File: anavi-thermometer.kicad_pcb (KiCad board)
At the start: 2 copper layers, 74.9 x 40.6 mm, 25 parts, among them P1 CONN_01X03, SW1 SW_DIP_x01, U1 I2C_SENS_1, U2 I2C_SENS_1, U3 I2C_SENS_1, U4 Conn_01x04

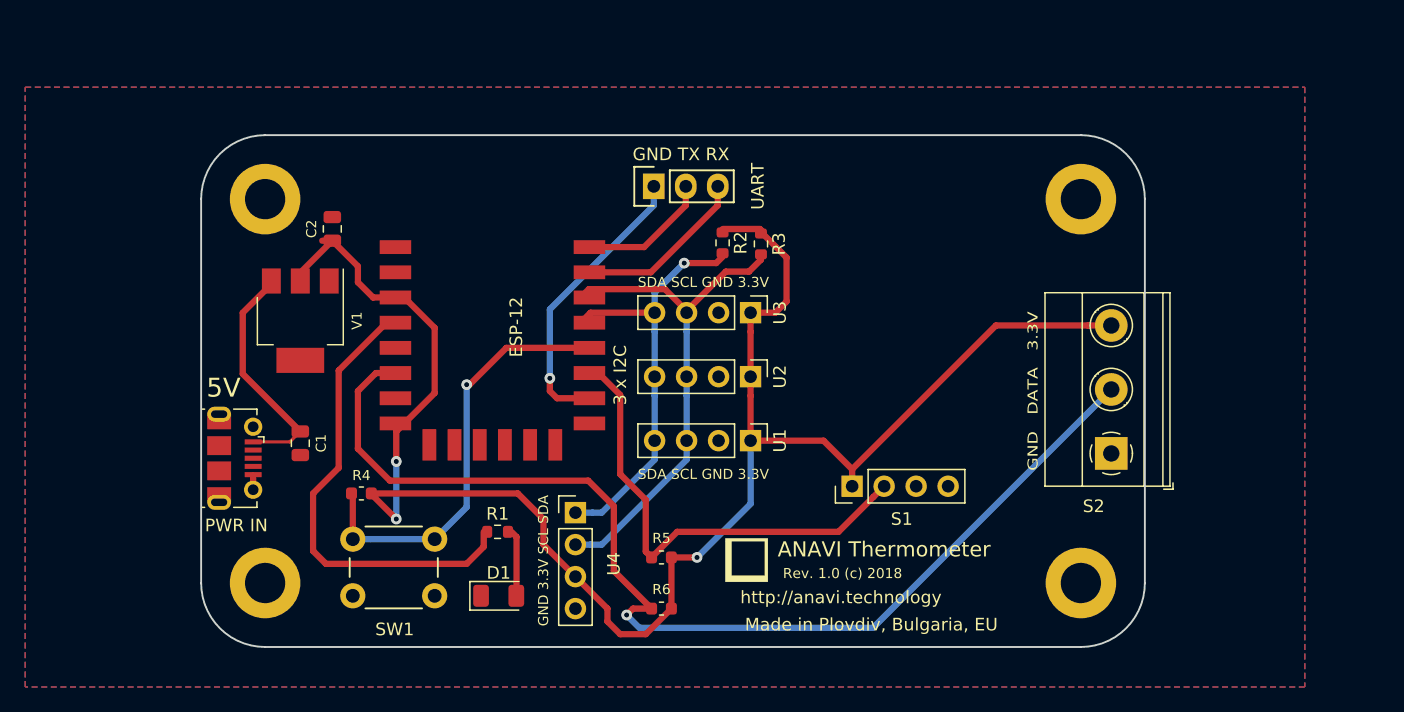
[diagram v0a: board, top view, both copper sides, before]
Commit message: rev 0.1
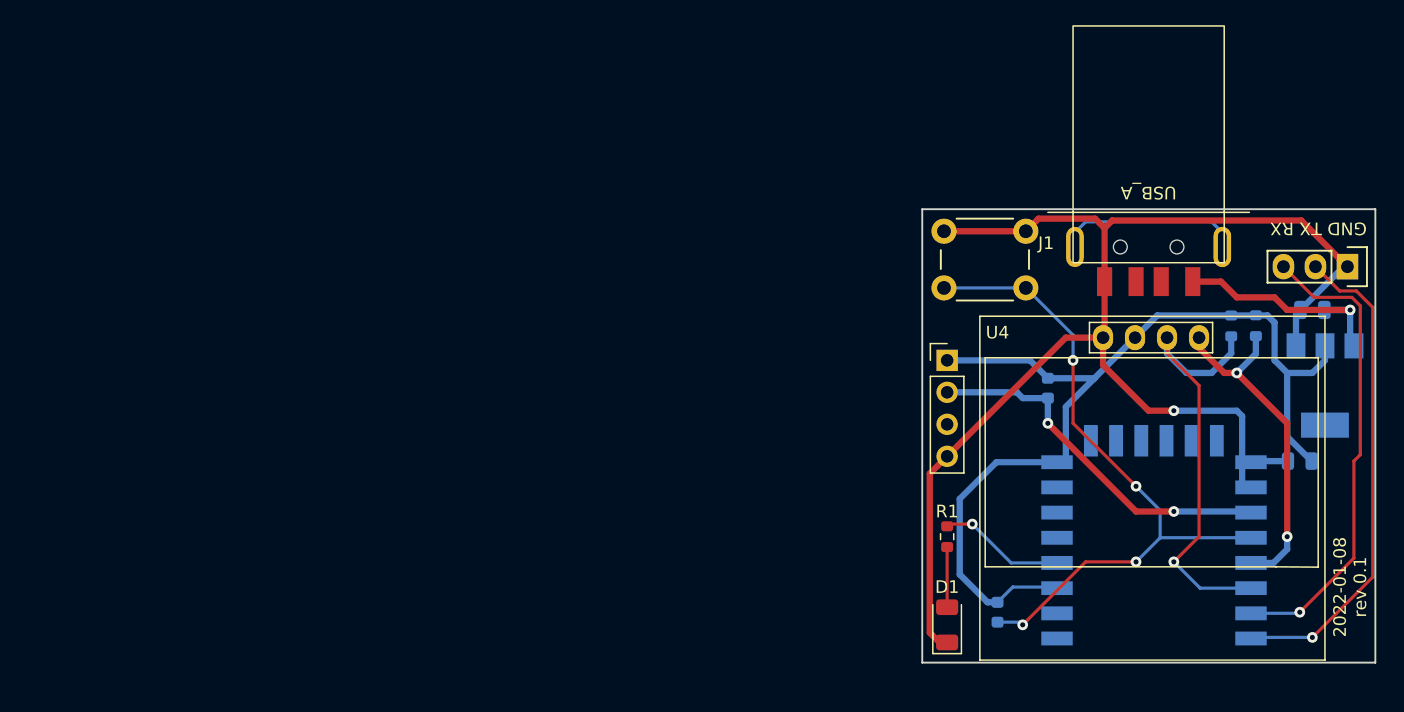
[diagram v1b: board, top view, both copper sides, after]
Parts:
- removed G***: LOGO, logo:anavi-logo
- removed PWR IN: USB_B_Micro, Connector_USB:USB_Micro-B_Molex-105017-0001
- removed R6: 4,7K, Resistor_SMD:R_0603_1608Metric
- removed REF** (x4): MountingHole_3.2mm_M3_DIN965_Pad, Mounting_Holes:MountingHole_3.2mm_M3_DIN965_Pad
- removed S2: DS18B20, TerminalBlock_Phoenix:TerminalBlock_Phoenix_MKDS-1,5-3-5.08_1x03_P5.08mm_Horizontal
- removed U1, U2, U3: I2C_SENS_1, Connector_PinHeader_2.54mm:PinHeader_1x04_P2.54mm_Vertical
- added J1: USB_A, GCT_USB1061_Horizontal:USB_A_Plug_GCT_USB1061_Horizontal, F.Cu at (140.0, 80.0)
- C1, C2, ESP-12, R2, R3, R4, R5, V1: moved to B.Cu
- U4: value Conn_01x04 -> SSD1306; footprint Connector_PinHeader_2.54mm:PinHeader_1x04_P2.54mm_Vertical -> SSD1306:128x64OLED
- moved V1 81.5 mm to (154.0, 91.0)
- moved C1 81.0 mm to (153.0, 85.0), turned to 180 degrees
- moved C2 79.0 mm to (152.0, 97.0), turned to 180 degrees
- moved ESP-12 61.0 mm to (133.4, 111.1)
- moved P1 55.4 mm to (155.8, 81.6), turned to -90 degrees
- moved R4 51.4 mm to (128.0, 109.0), turned to 90 degrees
- moved SW1 49.7 mm to (123.8, 78.8), turned to 0 degrees
- moved U4 45.6 mm to (140.0, 97.8)
- moved R2 42.9 mm to (148.5, 86.3)
- moved R3 37.9 mm to (146.6, 86.3)
- moved R1 35.7 mm to (124.0, 103.0), turned to -90 degrees
- moved D1 35.7 mm to (124.0, 110.0), turned to 90 degrees
- moved R5 33.5 mm to (132.0, 91.2), turned to -90 degrees
- moved S1 12.5 mm to (124.0, 89.0), turned to 0 degrees
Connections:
- ESP-12 pad 6: Net-(ESP-12-Pad6) -> unconnected-(ESP-12-Pad6)
- U4 pad 1: Net-(ESP-12-Pad13) -> GND
- U4 pad 2: Net-(ESP-12-Pad14) -> +3V3
- U4 pad 3: +3V3 -> Net-(ESP-12-Pad14)
- U4 pad 4: GND -> Net-(ESP-12-Pad13)
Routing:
- net Net-(ESP-12-Pad6): track 89.4 -> 0.00 mm, vias 1 -> 0
- net GND: track 23.5 -> 108.2 mm
- net +3V3: track 143.2 -> 78.8 mm, vias 3 -> 0
- net Net-(ESP-12-Pad16): track 11.2 -> 39.7 mm, vias 0 -> 1
- net Net-(ESP-12-Pad4): track 37.7 -> 10.8 mm, vias 0 -> 1
- net Net-(ESP-12-Pad15): track 14.6 -> 38.3 mm, vias 0 -> 1
- net Net-(ESP-12-Pad12): track 33.7 -> 53.1 mm, vias 2 -> 4
- net unconnected-(J1-Pad5): track 0.00 -> 14.7 mm
- net Net-(ESP-12-Pad11): track 38.6 -> 28.6 mm, vias 0 -> 2
- net Net-(ESP-12-Pad13): track 34.4 -> 27.9 mm, vias 1 -> 2
- net Net-(ESP-12-Pad14): track 40.6 -> 35.0 mm, vias 0 -> 1
- net +5V: track 19.4 -> 18.5 mm, vias 0 -> 1
- removed copper zone on B.Cu, net GND
- removed copper zone on F.Cu, net GND
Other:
- board size 74.9 x 40.6 mm -> 36 x 36 mm
- board text added: "2022-01-08 rev 0.1"
- board text added: "3V3"
- board text added: "DAT"
- board text added: "GND"
- board text added: "NC"
- board text added: "SDA SCL 3.3V GND"
- board text added: "based on Anavi thermometer"
- board text removed: "3 x I2C"
- board text removed: "5V"
- board text removed: "ANAVI Thermometer"
- board text removed: "GND 3.3V SCL SDA"
- board text removed: "GND DATA 3.3V"
- board text removed: "Made in Plovdiv, Bulgaria, EU"
- board text removed: "Rev. 1.0 (c) 2018"
- board text removed: "SDA SCL GND 3.3V"
- board text removed: "UART"
- board text removed: "http://anavi.technology"
